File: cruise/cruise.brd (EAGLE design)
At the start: 75.2 x 58.4 mm, 100 parts, among them IC1 24C04ASM, IC3 LD117AS33TR, Q1 AO4300, Q2 AO4300, Q3 AO4300, Q4 8MHz, U1 STM32F103CBT6, X5 SWD, X6 I2C

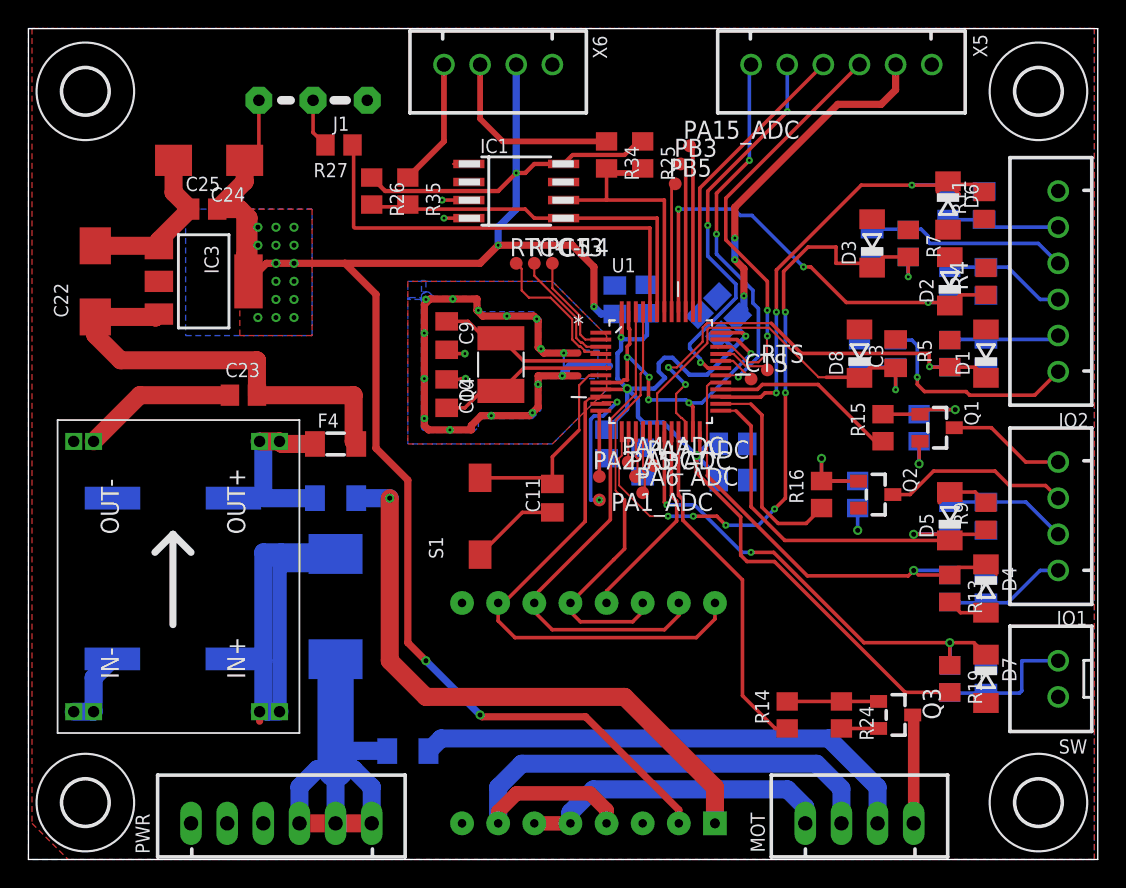
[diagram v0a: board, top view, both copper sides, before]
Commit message: Update cruise.brd
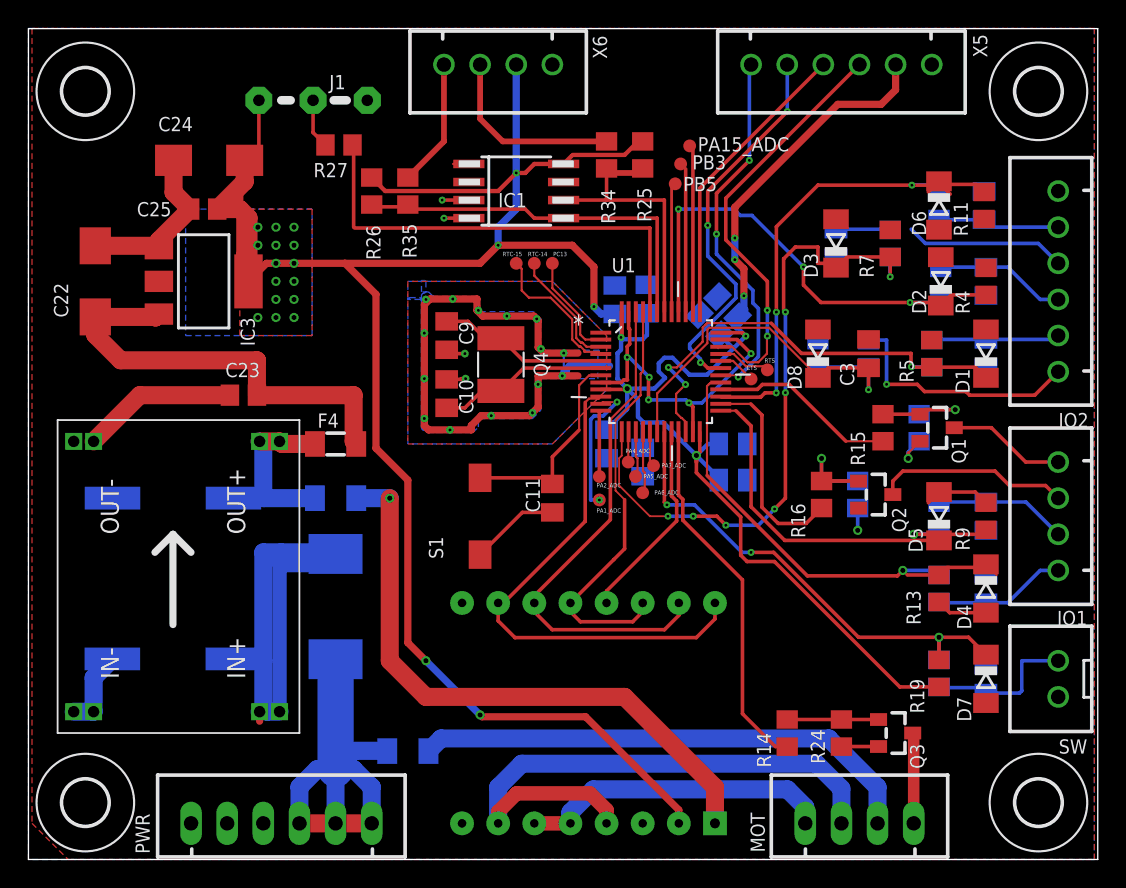
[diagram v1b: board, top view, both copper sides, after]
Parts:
- moved D8 2.92 mm to (55.5, 35.6)
- moved R21 2.92 mm to (55.5, 35.6)
- moved C4 2.54 mm to (56.8, 43.3)
- moved D3 2.54 mm to (56.8, 43.3)
- moved C3 1.91 mm to (59.1, 35.6)
- moved R20 1.91 mm to (59.1, 35.6)
- moved Q3 1.27 mm to (61.0, 8.89)
- moved R14 1.27 mm to (53.3, 8.89)
- moved R24 1.27 mm to (57.1, 8.89)
- moved R2 1.27 mm to (63.5, 35.6)
- moved R5 1.27 mm to (63.5, 35.6)
- moved R6 1.27 mm to (60.6, 43.3)
- moved R7 1.27 mm to (60.6, 43.3)
- moved R18 0.85 mm to (64.0, 13.1)
- moved R19 0.85 mm to (64.0, 13.1)
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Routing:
- net TPS_IN: track 15.3 -> 17.4 mm
- net OD_IN_LIGHT_PB12: track 31.8 -> 30.3 mm
- net GND: track 119.0 -> 120.4 mm
- net TIM3_CH2_SPD: track 34.4 -> 35.8 mm
- net PB10_OUT_SOLENOID: track 24.5 -> 25.8 mm
- net N$1: track 7.65 -> 6.38 mm
- net RPM_IN: track 7.75 -> 9.02 mm
- net IDLE_IN_PB14: track 35.4 -> 36.5 mm
- net VCC: track 241.6 -> 240.7 mm
- net SW_IN: track 9.81 -> 10.7 mm
- net STOP_IN: track 14.7 -> 15.5 mm
- net D_IN: track 8.96 -> 9.72 mm
- net OD_IN_L: track 8.58 -> 9.34 mm
- net STOP_IN_PA3: track 47.4 -> 46.6 mm
- net TPS_ADC: track 30.0 -> 29.3 mm
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
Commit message: схема
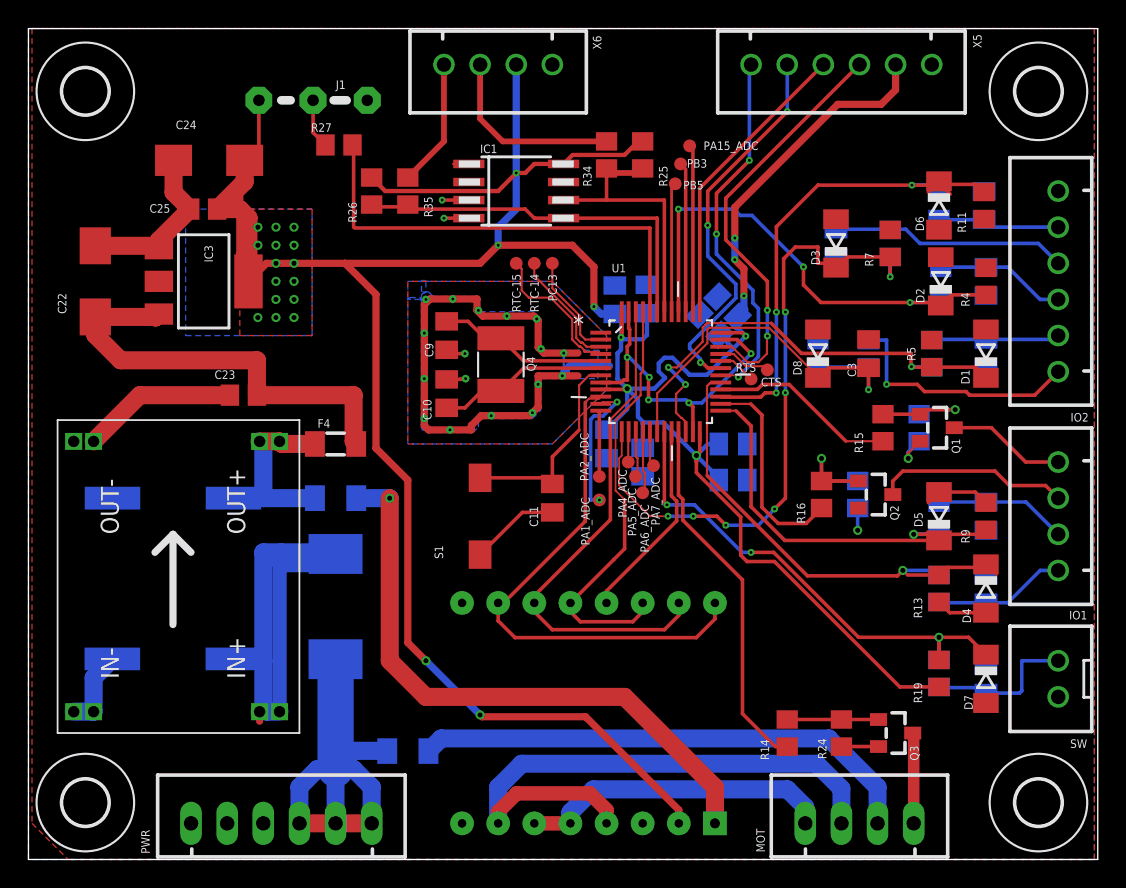
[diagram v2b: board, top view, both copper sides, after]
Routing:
- net STOP_IN: track 15.5 -> 17.0 mm
